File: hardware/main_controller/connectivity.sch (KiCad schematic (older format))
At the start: 16 parts

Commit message: Peripherals
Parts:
- removed JP?: Jumper, symbol Device:Jumper
- added J? (x2): Conn_01x08, symbol Connector_Generic:Conn_01x08
- added J? (x2): Conn_02x08_Odd_Even, symbol Connector_Generic:Conn_02x08_Odd_Even
- added J?: Conn_01x04, symbol Connector_Generic:Conn_01x04
- added J?: Conn_01x06, symbol Connector_Generic:Conn_01x06
- added J?: Conn_02x03_Counter_Clockwise, symbol Connector_Generic:Conn_02x03_Counter_Clockwise
- added J? (x2): RJ45, symbol Connector:RJ45
- added JP? (x3): Jumper_NO_Small, symbol Device:Jumper_NO_Small
- added R?: 4.7k, symbol Device:R
- added R?: 120, symbol Device:R
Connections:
- net labels added: CAN_H, CAN_L, CAN_PWR, CAN_RX, CAN_TX, GPIO_PE0, GPIO_PE1, GPIO_PE10, GPIO_PE11, GPIO_PE12, GPIO_PE13, GPIO_PE14, GPIO_PE15, GPIO_PE2, GPIO_PE3, GPIO_PE4, GPIO_PE5, GPIO_PE6, GPIO_PE7, GPIO_PE8, GPIO_PE9, I2C_SCL, I2C_SDA, SPI_CS1, SPI_CS2, SPI_CS3, SPI_MISO, SPI_MOSI, SPI_SCK
- wire segments 71 -> 219
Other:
- note added: "CAN"
- note added: "Deliver/Retrieve Power from CAN bus"
- note added: "GPIO"
- note added: "I2C"
- note added: "Optional CAN bus\ntermination resistor"
- note added: "SPI"
- moved on the sheet: C?, U?

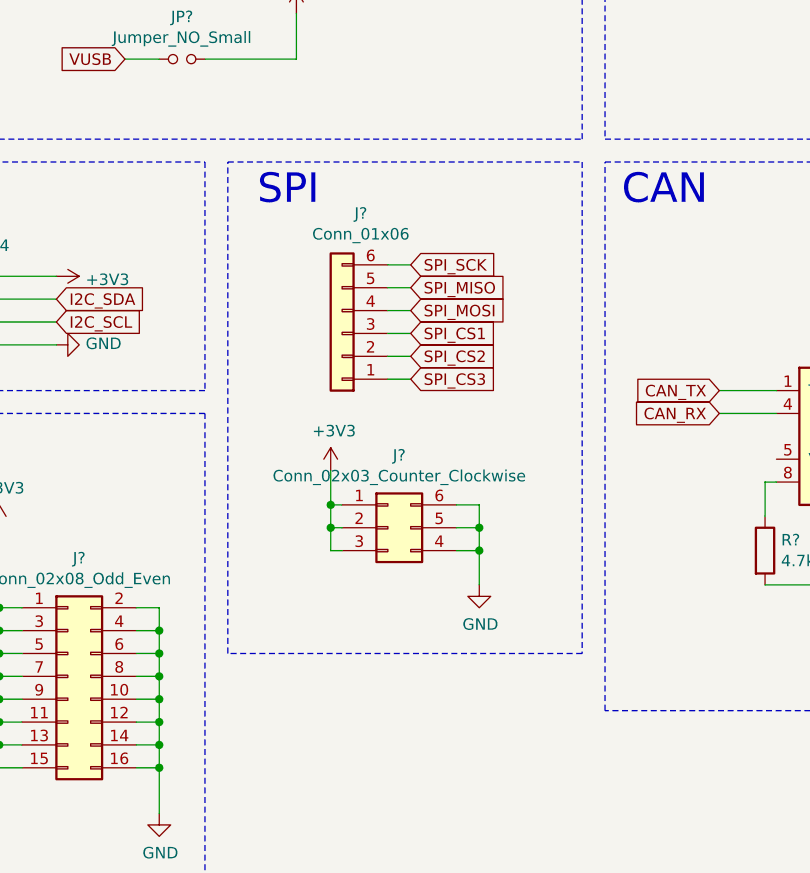
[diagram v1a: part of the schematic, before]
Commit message: LEDs
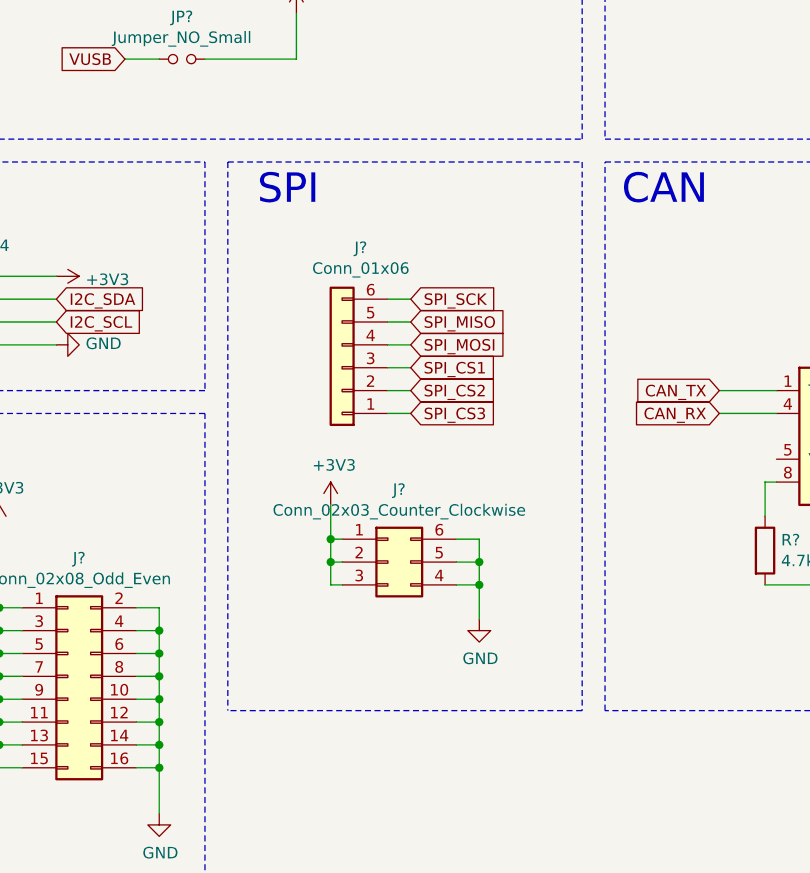
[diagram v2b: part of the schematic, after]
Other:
- moved on the sheet: J?
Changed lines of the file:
@@
 L Connector_Generic:Conn_01x06 J?
 U 1 1 5FF94D26
-P 4650 4050
-F 0 "J?" H 4568 3525 50  0000 C CNN
-F 1 "Conn_01x06" H 4568 3616 50  0000 C CNN
-F 2 "" H 4650 4050 50  0001 C CNN
-F 3 "~" H 4650 4050 50  0001 C CNN
-	1    4650 4050
+P 4650 4200
+F 0 "J?" H 4568 3675 50  0000 C CNN
+F 1 "Conn_01x06" H 4568 3766 50  0000 C CNN
+F 2 "" H 4650 4200 50  0001 C CNN
+F 3 "~" H 4650 4200 50  0001 C CNN
+	1    4650 4200
 	-1   0    0    1
 $EndComp
 Wire Wire Line
-	4850 3750 4950 3750
-Wire Wire Line
-	4850 3850 4950 3850
-Wire Wire Line
-	4850 3950 4950 3950
-Wire Wire Line
-	4850 4050 4950 4050
-Wire Wire Line
-	4850 4150 4950 4150
-Wire Wire Line
-	4850 4250 4950 4250
-Text GLabel 4950 3750 2    50   Input ~ 0
+	4850 3900 4950 3900
+Wire Wire Line
+	4850 4000 4950 4000
+Wire Wire Line
+	4850 4100 4950 4100
+Wire Wire Line
+	4850 4200 4950 4200
+Wire Wire Line
+	4850 4300 4950 4300
+Wire Wire Line
+	4850 4400 4950 4400
+Text GLabel 4950 3900 2    50   Input ~ 0
 SPI_SCK
-Text GLabel 4950 3850 2    50   Input ~ 0
+Text GLabel 4950 4000 2    50   Input ~ 0
 SPI_MISO
-Text GLabel 4950 3950 2    50   Input ~ 0
+Text GLabel 4950 4100 2    50   Input ~ 0
 SPI_MOSI
-Text GLabel 4950 4050 2    50   Input ~ 0
+Text GLabel 4950 4200 2    50   Input ~ 0
 SPI_CS1
-Text GLabel 4950 4150 2    50   Input ~ 0
+Text GLabel 4950 4300 2    50   Input ~ 0
 SPI_CS2
-Text GLabel 4950 4250 2    50   Input ~ 0
+Text GLabel 4950 4400 2    50   Input ~ 0
 SPI_CS3
 $Comp
 L Connector_Generic:Conn_02x03_Counter_Clockwise J?
 U 1 1 5FFE4E2A
-P 4850 4900
-F 0 "J?" H 4900 5217 50  0000 C CNN
-F 1 "Conn_02x03_Counter_Clockwise" H 4900 5126 50  0000 C CNN
-F 2 "" H 4850 4900 50  0001 C CNN
-F 3 "~" H 4850 4900 50  0001 C CNN
-	1    4850 4900
+P 4850 5050
+F 0 "J?" H 4900 5367 50  0000 C CNN
+F 1 "Conn_02x03_Counter_Clockwise" H 4900 5276 50  0000 C CNN
+F 2 "" H 4850 5050 50  0001 C CNN
+F 3 "~" H 4850 5050 50  0001 C CNN
+	1    4850 5050
 	1    0    0    -1
 $EndComp
@@
 L power:+3V3 #PWR?
 U 1 1 5FFE6348
-P 4600 4650
-F 0 "#PWR?" H 4600 4500 50  0001 C CNN
-F 1 "+3V3" H 4615 4823 50  0000 C CNN
-F 2 "" H 4600 4650 50  0001 C CNN
-F 3 "" H 4600 4650 50  0001 C CNN
-	1    4600 4650
+P 4600 4800
+F 0 "#PWR?" H 4600 4650 50  0001 C CNN
+F 1 "+3V3" H 4615 4973 50  0000 C CNN
+F 2 "" H 4600 4800 50  0001 C CNN
+F 3 "" H 4600 4800 50  0001 C CNN
+	1    4600 4800
 	1    0    0    -1
 $EndComp
@@
 L power:GND #PWR?
 U 1 1 5FFE73F3
-P 5250 5150
-F 0 "#PWR?" H 5250 4900 50  0001 C CNN
-F 1 "GND" H 5255 4977 50  0000 C CNN
-F 2 "" H 5250 5150 50  0001 C CNN
-F 3 "" H 5250 5150 50  0001 C CNN
-	1    5250 5150
-	1    0    0    -1
-$EndComp
-Wire Wire Line
-	5150 4800 5250 4800
-Wire Wire Line
-	5250 4800 5250 4900
-Wire Wire Line
-	5150 4900 5250 4900
-Connection ~ 5250 4900
-Wire Wire Line
-	5250 4900 5250 5000
-Wire Wire Line
-	5250 5000 5150 5000
-Connection ~ 5250 5000
-Wire Wire Line
-	5250 5000 5250 5150
-Wire Wire Line
-	4650 4800 4600 4800
-Wire Wire Line
-	4600 4800 4600 4650
-Wire Wire Line
-	4650 5000 4600 5000
-Wire Wire Line
-	4600 5000 4600 4900
-Connection ~ 4600 4800
-Wire Wire Line
-	4650 4900 4600 4900
-Connection ~ 4600 4900
-Wire Wire Line
-	4600 4900 4600 4800
+P 5250 5300
+F 0 "#PWR?" H 5250 5050 50  0001 C CNN
+F 1 "GND" H 5255 5127 50  0000 C CNN
+F 2 "" H 5250 5300 50  0001 C CNN
+F 3 "" H 5250 5300 50  0001 C CNN
+	1    5250 5300
+	1    0    0    -1
+$EndComp
+Wire Wire Line
+	5150 4950 5250 4950
+Wire Wire Line
+	5250 4950 5250 5050
+Wire Wire Line
+	5150 5050 5250 5050
+Connection ~ 5250 5050
+Wire Wire Line
+	5250 5050 5250 5150
+Wire Wire Line
+	5250 5150 5150 5150
+Connection ~ 5250 5150
+Wire Wire Line
+	5250 5150 5250 5300
+Wire Wire Line
+	4650 4950 4600 4950
+Wire Wire Line
+	4600 4950 4600 4800
+Wire Wire Line
+	4650 5150 4600 5150
+Wire Wire Line
+	4600 5150 4600 5050
+Connection ~ 4600 4950
+Wire Wire Line
+	4650 5050 4600 5050
+Connection ~ 4600 5050
+Wire Wire Line
+	4600 5050 4600 4950
 Wire Notes Line
 	4150 3300 5700 3300
-Wire Notes Line
-	5700 3300 5700 5450
-Wire Notes Line
-	5700 5450 4150 5450
-Wire Notes Line
-	4150 5450 4150 3300
 Text Notes 4550 3500 2    129  ~ 0
 SPI
@@
 Text Notes 7250 3450 0    50   ~ 0
 Deliver/Retrieve Power from CAN bus
+Wire Notes Line
+	5700 5700 4150 5700
+Wire Notes Line
+	5700 3300 5700 5700
+Wire Notes Line
+	4150 3300 4150 5700
 $EndSCHEMATC
